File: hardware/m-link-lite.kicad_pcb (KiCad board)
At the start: 2 copper layers, 24 x 30 mm, 22 parts, among them J1 ADC IN, J2 PROGRAM, J3 SIG, SW1 DTR, U1 AP1117-33, U3 74LS365, U4 ESP-12F

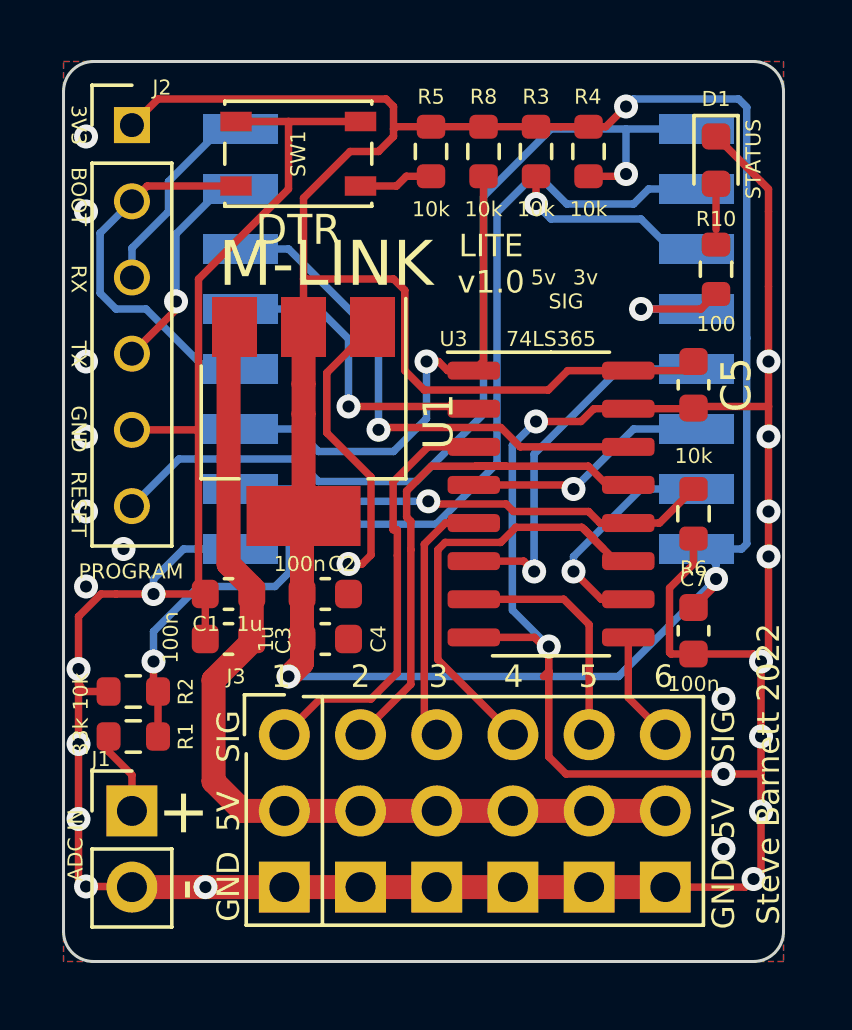
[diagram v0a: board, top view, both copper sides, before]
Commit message: Rework v1.2 layout.
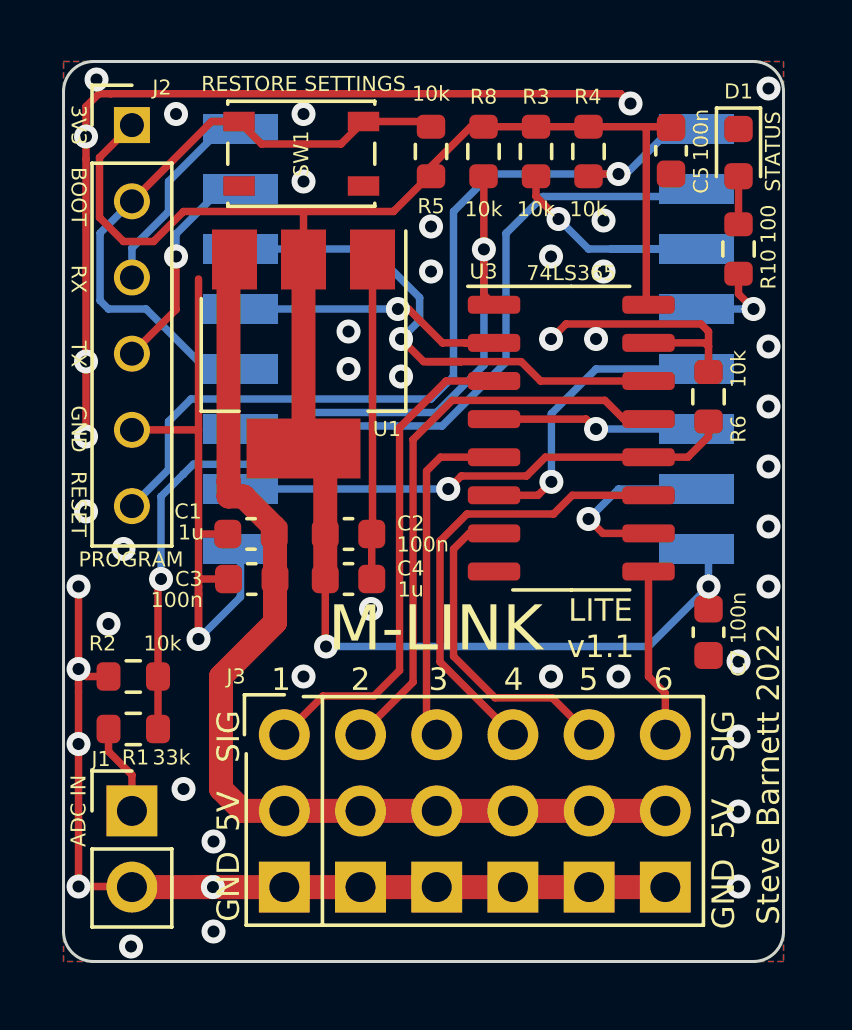
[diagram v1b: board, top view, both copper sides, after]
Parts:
- SW1: value DTR -> RESTORE SETTINGS
- moved C5 7.84 mm to (99.2, 72.0)
- moved R6 3.93 mm to (100.5, 80.2), turned to 90 degrees
- moved U3 2.30 mm to (95.9, 81.6)
- moved U1 2.25 mm to (87.0, 78.8)
- moved C2 2.14 mm to (88.5, 84.8)
- moved C3 2.14 mm to (85.3, 86.2)
- moved C4 2.14 mm to (88.5, 86.2)
- moved C1 2.14 mm to (85.2, 84.8)
- moved R10 1.01 mm to (101.5, 75.2)
- moved D1 0.79 mm to (101.5, 72.0)
- moved C7 0.50 mm to (100.5, 88.0)
- moved R2 0.50 mm to (81.3, 89.5)
- moved R1 0.25 mm to (81.3, 91.2)
- moved SW1 0.10 mm to (86.9, 72.1), turned to 180 degrees
- turned R5 to 90 degrees
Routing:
- net GND: track 139.8 -> 101.6 mm, vias 27 -> 45
- net +3V3: track 93.8 -> 61.3 mm, vias 3 -> 2
- net /DTR: track 15.4 -> 21.1 mm
- net /CH3: track 8.46 -> 12.0 mm
- net +5V: track 31.4 -> 34.5 mm
- net /CH5: track 7.87 -> 10.7 mm
- net /CH5_LV: track 12.7 -> 9.83 mm
- net /RESET: track 31.9 -> 29.2 mm
- net /EN: track 6.90 -> 9.60 mm
- net /CH1: track 14.3 -> 16.6 mm
- net /CH6: track 3.76 -> 5.67 mm
- net /ADC: track 34.1 -> 32.4 mm
- net /CH6_LV: track 7.74 -> 6.21 mm
- net /CH3_LV: track 8.31 -> 6.89 mm
- net /LED1: track 4.56 -> 3.28 mm
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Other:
- board text added: "LITE v1.1"
- board text removed: "+"
- board text removed: "-"
- board text removed: "3v"
- board text removed: "5v"
- board text removed: "LITE v1.0"
